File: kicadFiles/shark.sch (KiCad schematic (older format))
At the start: 262 parts, among them J1 USB_C_Receptacle, J2 Conn_01x04_Male, J3 Conn_01x04_Male, J4 Conn_01x04_Male, Q1 AO4406AL, SW1 MXSwitch, SW10 MXSwitch, SW11 MXSwitch, SW12 MXSwitch, SW13 MXSwitch, SW14 MXSwitch, SW15 MXSwitch, SW16 MXSwitch, SW17 MXSwitch, SW18 MXSwitch, SW19 MXSwitch, SW2 MXSwitch, SW20 MXSwitch, SW21 MXSwitch, SW22 MXSwitch, SW23 MXSwitch, SW24 MXSwitch, SW25 MXSwitch, SW26 MXSwitch, SW27 MXSwitch, SW28 MXSwitch, SW29 MXSwitch, SW3 MXSwitch, SW30 MXSwitch, SW31 MXSwitch, SW32 MXSwitch, SW33 MXSwitch, SW34 MXSwitch, SW35 MXSwitch, SW36 MXSwitch, SW37 MXSwitch, SW38 MXSwitch, SW39 MXSwitch, SW4 MXSwitch, SW40 MXSwitch, SW41 MXSwitch, SW42 MXSwitch, SW43 MXSwitch, SW44 MXSwitch, SW45 MXSwitch, SW46 MXSwitch, SW47 MXSwitch, SW48 MXSwitch, SW49 MXSwitch, SW5 MXSwitch, SW50 MXSwitch, SW51 MXSwitch, SW6 MXSwitch, SW7 MXSwitch, SW8 MXSwitch, SW9 MXSwitch, U1 STM32F303CCT6, U2 MCP1700-3302E_SOT23, Y1 8MHz

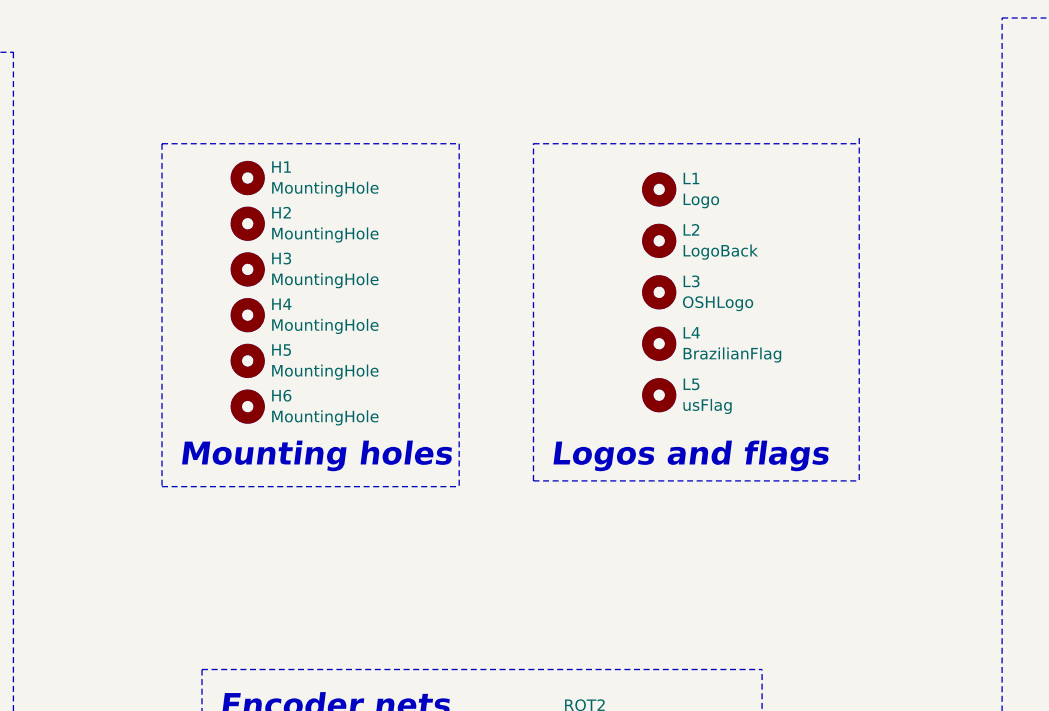
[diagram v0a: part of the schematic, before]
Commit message: [Feature] Adde the Acheron Project logo
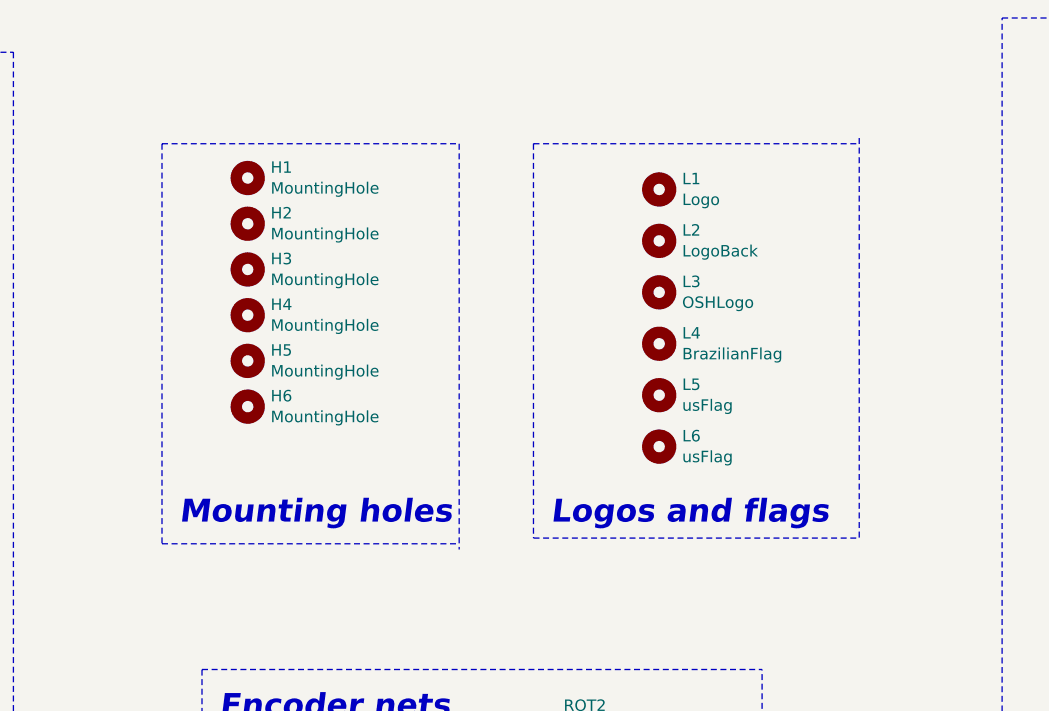
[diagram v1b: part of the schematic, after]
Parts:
- added L6: usFlag, acheronLogos:acheronLogo, symbol Mechanical:MountingHole
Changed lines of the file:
@@
 Wire Wire Line
 	5900 12800 6175 12800
-Text Notes 14925 4425 0    100  Italic 20
+Text Notes 14925 4675 0    100  Italic 20
 Mounting holes
-Wire Notes Line width 20
-	16475 4475 16475 3000
-Text Notes 16550 4425 0    100  Italic 20
+Text Notes 16550 4675 0    100  Italic 20
 Logos and flags
 Wire Notes Line width 20
@@
 USB Connector
 Wire Notes Line width 20
-	14850 3000 14850 4500
-Wire Notes Line width 20
-	16150 3000 16150 4500
-Wire Notes Line width 20
-	14850 4500 16150 4500
+	14850 4750 16150 4750
 Wire Notes Line width 20 style dash_dot
 	14850 3000 16150 3000
@@
 	16475 3000 17900 3000
 Wire Notes Line width 20
-	17900 2975 17900 4475
-Wire Notes Line width 20
-	16475 4475 17900 4475
+	16475 4725 17900 4725
 Wire Notes Line width 20
 	15025 7125 17425 7125
@@
 Text GLabel 13400 10950 2    50   Input ~ 0
 Extra8
+Wire Notes Line width 20
+	14850 3000 14850 4750
+Wire Notes Line width 20
+	16150 3000 16150 4775
+$Comp
+L Mechanical:MountingHole L6
+U 1 1 5D02D130
+P 17025 4325
+F 0 "L6" H 17125 4371 50  0000 L CNN
+F 1 "usFlag" H 17125 4280 50  0000 L CNN
+F 2 "acheronLogos:acheronLogo" H 17025 4325 50  0001 C CNN
+F 3 "~" H 17025 4325 50  0001 C CNN
+	1    17025 4325
+	1    0    0    -1
+$EndComp
+Wire Notes Line width 20
+	16475 3000 16475 4725
+Wire Notes Line width 20
+	17900 2975 17900 4725
 $EndSCHEMATC

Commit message: [Update] Enlarged the plate pegs holes in the PCB
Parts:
- J1: symbol Connector:USB_C_Receptacle -> shark-rescue:USB_C_Receptacle-Connector
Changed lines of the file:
@@
 EESchema Schematic File Version 4
 LIBS:shark-cache
-EELAYER 26 0
+EELAYER 29 0
 EELAYER END
 $Descr A2 23386 16535
@@
 Title "SharkPCB"
 Date "2019-03-20"
-Rev "3.1.6"
+Rev "3.1.7"
 Comp "Gondolin Electronics"
 Comment1 ""
@@
 	16025 9850 16250 9850
 $Comp
-L Connector:USB_C_Receptacle J1
+L shark-rescue:USB_C_Receptacle-Connector J1
 U 1 1 5CC01BA3
 P 8625 10675
